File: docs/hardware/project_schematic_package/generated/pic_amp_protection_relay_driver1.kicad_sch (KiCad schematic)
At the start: 1 part, among them U3 ULN2803A

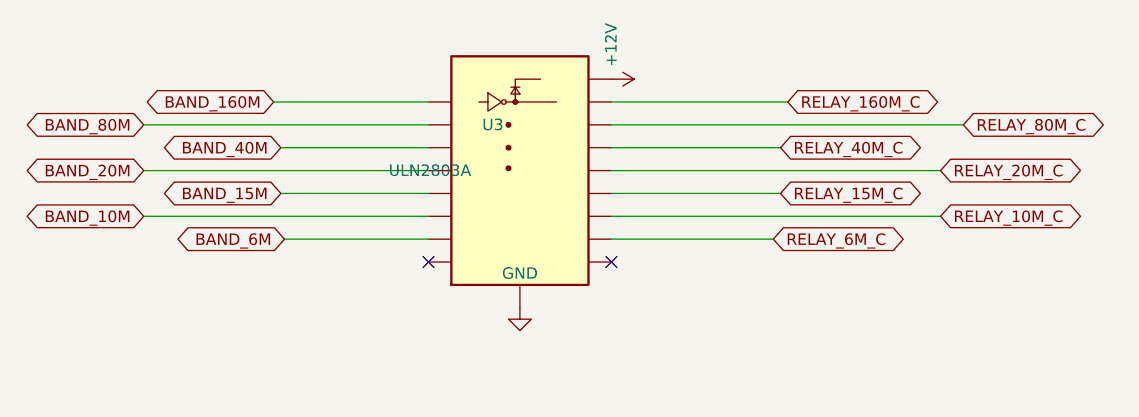
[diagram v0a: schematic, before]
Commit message: Add structured schematic generation rules
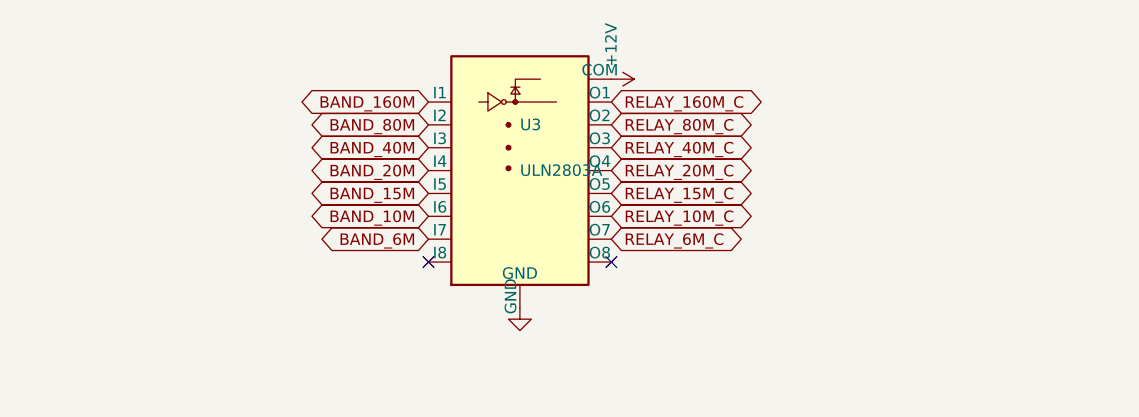
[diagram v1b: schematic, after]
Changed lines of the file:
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@@
     (fields_autoplaced yes)
     (property "Reference" "U3"
-      (at 140.510 93.980 0)
-      (effects
-        (font
-          (size 1.27 1.27))))
+      (at 143.51 93.97999999999999 0)
+      (effects
+        (font
+          (size 1.27 1.27))
+        (justify left)))
     (property "Value" "ULN2803A"
-      (at 133.510 99.060 0)
-      (effects
-        (font
-          (size 1.27 1.27))))
+      (at 143.51 99.06 0)
+      (effects
+        (font
+          (size 1.27 1.27))
+        (justify left)))
     (property "Footprint" "Package_DIP:DIP-18_W7.62mm"
       (at 143.51 96.52 0)
@@
     (instances
       (project "SKiDL-Generated"
-        (path "/12796df2-447d-4449-8763-29ebc11da552/1515956d-950e-50fb-a850-78278e328eb4"
+        (path "/d61bc15e-84d8-4f6a-aa49-f72cca060f2c/1515956d-950e-50fb-a850-78278e328eb4"
           (reference "U3")
           (unit 1)))))
   (global_label "BAND_160M"
     (shape bidirectional)
-    (at 116.150 91.440 180)
+    (at 133.35 91.44 180)
     (effects
       (font
@@
   (global_label "BAND_80M"
     (shape bidirectional)
-    (at 101.710 93.980 180)
+    (at 133.35 93.98 180)
     (effects
       (font
@@
   (global_label "BAND_40M"
     (shape bidirectional)
-    (at 116.950 96.520 180)
+    (at 133.35 96.52 180)
     (effects
       (font
@@
   (global_label "BAND_20M"
     (shape bidirectional)
-    (at 101.710 99.060 180)
+    (at 133.35 99.06 180)
     (effects
       (font
@@
   (global_label "BAND_15M"
     (shape bidirectional)
-    (at 116.950 101.600 180)
+    (at 133.35 101.6 180)
     (effects
       (font
@@
   (global_label "BAND_10M"
     (shape bidirectional)
-    (at 101.710 104.140 180)
+    (at 133.35 104.14 180)
     (effects
       (font
@@
   (global_label "BAND_6M"
     (shape bidirectional)
-    (at 117.350 106.680 180)
+    (at 133.35 106.68 180)
     (effects
       (font
@@
     (dnp no)
     (fields_autoplaced yes)
-    (property "Reference" "#PWR017"
+    (property "Reference" "#PWR020"
       (at 143.51 113.03 0)
       (effects
@@
       (project "SKiDL-Generated"
         (path "/218b5f90-a139-55d3-a988-331ecbe7ee0c"
-          (reference "#PWR017")
+          (reference "#PWR020")
           (unit 1)))))
   (symbol
@@
     (dnp no)
     (fields_autoplaced yes)
-    (property "Reference" "#PWR018"
+    (property "Reference" "#PWR021"
       (at 153.67 87.63000000000001 0)
       (effects
@@
       (project "SKiDL-Generated"
         (path "/218b5f90-a139-55d3-a988-331ecbe7ee0c"
-          (reference "#PWR018")
+          (reference "#PWR021")
           (unit 1)))))
   (global_label "RELAY_160M_C"
     (shape bidirectional)
-    (at 173.270 91.440 0)
+    (at 153.67 91.44 0)
     (effects
       (font
@@
   (global_label "RELAY_80M_C"
     (shape bidirectional)
-    (at 192.790 93.980 0)
+    (at 153.67 93.98 0)
     (effects
       (font
@@
   (global_label "RELAY_40M_C"
     (shape bidirectional)
-    (at 172.470 96.520 0)
+    (at 153.67 96.52 0)
     (effects
       (font
@@
   (global_label "RELAY_20M_C"
     (shape bidirectional)
-    (at 190.250 99.060 0)
+    (at 153.67 99.06 0)
     (effects
       (font
@@
   (global_label "RELAY_15M_C"
     (shape bidirectional)
-    (at 172.470 101.600 0)
+    (at 153.67 101.6 0)
     (effects
       (font
@@
   (global_label "RELAY_10M_C"
     (shape bidirectional)
-    (at 190.250 104.140 0)
+    (at 153.67 104.14 0)
     (effects
       (font
@@
   (global_label "RELAY_6M_C"
     (shape bidirectional)
-    (at 171.670 106.680 0)
+    (at 153.67 106.68 0)
     (effects
       (font
@@
   (no_connect
     (at 153.67 109.22)
-)
-  (wire
-    (pts
-      (xy 133.350 91.440)
-      (xy 116.150 91.440))
-    (stroke
-      (width 0)
-      (type default))
-)
-  (wire
-    (pts
-      (xy 133.350 93.980)
-      (xy 101.710 93.980))
-    (stroke
-      (width 0)
-      (type default))
-)
-  (wire
-    (pts
-      (xy 133.350 96.520)
-      (xy 116.950 96.520))
-    (stroke
-      (width 0)
-      (type default))
-)
-  (wire
-    (pts
-      (xy 133.350 99.060)
-      (xy 101.710 99.060))
-    (stroke
-      (width 0)
-      (type default))
-)
-  (wire
-    (pts
-      (xy 133.350 101.600)
-      (xy 116.950 101.600))
-    (stroke
-      (width 0)
-      (type default))
-)
-  (wire
-    (pts
-      (xy 133.350 104.140)
-      (xy 101.710 104.140))
-    (stroke
-      (width 0)
-      (type default))
-)
-  (wire
-    (pts
-      (xy 133.350 106.680)
-      (xy 117.350 106.680))
-    (stroke
-      (width 0)
-      (type default))
-)
-  (wire
-    (pts
-      (xy 153.670 91.440)
-      (xy 173.270 91.440))
-    (stroke
-      (width 0)
-      (type default))
-)
-  (wire
-    (pts
-      (xy 153.670 93.980)
-      (xy 192.790 93.980))
-    (stroke
-      (width 0)
-      (type default))
-)
-  (wire
-    (pts
-      (xy 153.670 96.520)
-      (xy 172.470 96.520))
-    (stroke
-      (width 0)
-      (type default))
-)
-  (wire
-    (pts
-      (xy 153.670 99.060)
-      (xy 190.250 99.060))
-    (stroke
-      (width 0)
-      (type default))
-)
-  (wire
-    (pts
-      (xy 153.670 101.600)
-      (xy 172.470 101.600))
-    (stroke
-      (width 0)
-      (type default))
-)
-  (wire
-    (pts
-      (xy 153.670 104.140)
-      (xy 190.250 104.140))
-    (stroke
-      (width 0)
-      (type default))
-)
-  (wire
-    (pts
-      (xy 153.670 106.680)
-      (xy 171.670 106.680))
-    (stroke
-      (width 0)
-      (type default))
-)
-)
+))

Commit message: Update schematic generation work
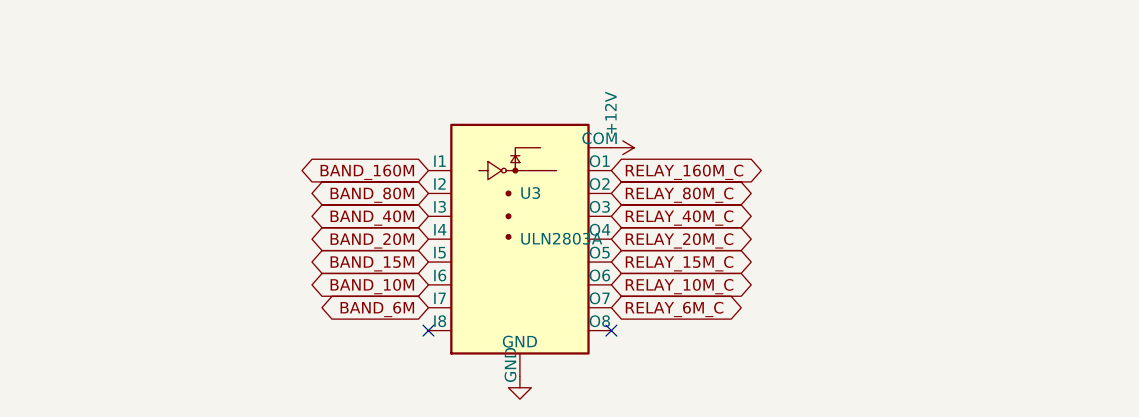
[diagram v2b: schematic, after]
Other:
- moved on the sheet: U3
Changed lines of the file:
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@@
   (symbol
     (lib_id "Transistor_Array:ULN2803A")
-    (at 143.51 96.52 0)
+    (at 143.51 104.14 0)
     (unit 1)
     (exclude_from_sim no)
@@
     (fields_autoplaced yes)
     (property "Reference" "U3"
-      (at 143.51 93.97999999999999 0)
+      (at 143.51 101.6 0)
       (effects
         (font
@@
         (justify left)))
     (property "Value" "ULN2803A"
-      (at 143.51 99.06 0)
+      (at 143.51 106.68 0)
       (effects
         (font
@@
         (justify left)))
     (property "Footprint" "Package_DIP:DIP-18_W7.62mm"
-      (at 143.51 96.52 0)
+      (at 143.51 104.14 0)
       (effects
         (font
@@
         (hide yes)))
     (property "Datasheet" "http://www.ti.com/lit/ds/symlink/uln2803a.pdf"
-      (at 143.51 96.52 0)
+      (at 143.51 104.14 0)
       (effects
         (font
@@
         (hide yes)))
     (property "Description" "Darlington Transistor Arrays, SOIC18/DIP18"
-      (at 143.51 96.52 0)
+      (at 143.51 104.14 0)
       (effects
         (font
@@
     (instances
       (project "SKiDL-Generated"
-        (path "/d61bc15e-84d8-4f6a-aa49-f72cca060f2c/1515956d-950e-50fb-a850-78278e328eb4"
+        (path "/1bbe9d5f-3fba-4b26-b038-cadb36f9032d/1515956d-950e-50fb-a850-78278e328eb4"
           (reference "U3")
           (unit 1)))))
   (global_label "BAND_160M"
     (shape bidirectional)
-    (at 133.35 91.44 180)
+    (at 133.35 99.06 180)
     (effects
       (font
@@
   (global_label "BAND_80M"
     (shape bidirectional)
-    (at 133.35 93.98 180)
+    (at 133.35 101.6 180)
     (effects
       (font
@@
   (global_label "BAND_40M"
     (shape bidirectional)
-    (at 133.35 96.52 180)
+    (at 133.35 104.14 180)
     (effects
       (font
@@
   (global_label "BAND_20M"
     (shape bidirectional)
-    (at 133.35 99.06 180)
+    (at 133.35 106.68 180)
     (effects
       (font
@@
   (global_label "BAND_15M"
     (shape bidirectional)
-    (at 133.35 101.6 180)
+    (at 133.35 109.22 180)
     (effects
       (font
@@
   (global_label "BAND_10M"
     (shape bidirectional)
-    (at 133.35 104.14 180)
+    (at 133.35 111.76 180)
     (effects
       (font
@@
   (global_label "BAND_6M"
     (shape bidirectional)
-    (at 133.35 106.68 180)
+    (at 133.35 114.3 180)
     (effects
       (font
@@
   (symbol
     (lib_id "power:GND")
-    (at 143.51 114.3 0.0)
+    (at 143.51 121.92 0.0)
     (unit 1)
     (exclude_from_sim yes)
@@
     (fields_autoplaced yes)
     (property "Reference" "#PWR020"
-      (at 143.51 113.03 0)
+      (at 143.51 120.65 0)
       (effects
         (font
@@
         (hide yes)))
     (property "Value" "GND"
-      (at 143.51 110.49 0)
+      (at 143.51 118.11 0)
       (effects
         (font
           (size 1.27 1.27))))
     (property "Footprint" ""
-      (at 143.51 114.3 0)
+      (at 143.51 121.92 0)
       (effects
         (font
@@
         (hide yes)))
     (property "Datasheet" ""
-      (at 143.51 114.3 0)
+      (at 143.51 121.92 0)
       (effects
         (font
@@
   (symbol
     (lib_id "power:+12V")
-    (at 153.67 88.9 270.0)
+    (at 153.67 96.52 270.0)
     (unit 1)
     (exclude_from_sim yes)
@@
     (fields_autoplaced yes)
     (property "Reference" "#PWR021"
-      (at 153.67 87.63000000000001 0)
+      (at 153.67 95.25 0)
       (effects
         (font
@@
         (hide yes)))
     (property "Value" "+12V"
-      (at 153.67 85.09 0)
+      (at 153.67 92.71 0)
       (effects
         (font
           (size 1.27 1.27))))
     (property "Footprint" ""
-      (at 153.67 88.9 0)
+      (at 153.67 96.52 0)
       (effects
         (font
@@
         (hide yes)))
     (property "Datasheet" ""
-      (at 153.67 88.9 0)
+      (at 153.67 96.52 0)
       (effects
         (font
@@
   (global_label "RELAY_160M_C"
     (shape bidirectional)
-    (at 153.67 91.44 0)
+    (at 153.67 99.06 0)
     (effects
       (font
@@
   (global_label "RELAY_80M_C"
     (shape bidirectional)
-    (at 153.67 93.98 0)
+    (at 153.67 101.6 0)
     (effects
       (font
@@
   (global_label "RELAY_40M_C"
     (shape bidirectional)
-    (at 153.67 96.52 0)
+    (at 153.67 104.14 0)
     (effects
       (font
@@
   (global_label "RELAY_20M_C"
     (shape bidirectional)
-    (at 153.67 99.06 0)
+    (at 153.67 106.68 0)
     (effects
       (font
@@
   (global_label "RELAY_15M_C"
     (shape bidirectional)
-    (at 153.67 101.6 0)
+    (at 153.67 109.22 0)
     (effects
       (font
@@
   (global_label "RELAY_10M_C"
     (shape bidirectional)
-    (at 153.67 104.14 0)
+    (at 153.67 111.76 0)
     (effects
       (font
@@
   (global_label "RELAY_6M_C"
     (shape bidirectional)
-    (at 153.67 106.68 0)
+    (at 153.67 114.3 0)
     (effects
       (font
@@
 )
   (no_connect
-    (at 133.35 109.22)
+    (at 133.35 116.84)
 )
   (no_connect
-    (at 153.67 109.22)
+    (at 153.67 116.84)
 ))
